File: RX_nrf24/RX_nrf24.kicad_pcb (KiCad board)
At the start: 2 copper layers, 58.5 x 26.2 mm, 44 parts, among them J1 USB_B_Micro, J2 Conn_01x03_Male, J3 Conn_Coaxial, J4 Conn_01x10_Male, J5 Conn_01x04_Female, J6 Conn_01x06_Male, J7 Conn_01x10_Male, J8 Conn_01x10_Male, SW1 SW_Push, U1 USBLC6-2SC6, U2 MCP1700-3302E_SOT23, U3 STM32F103C8Tx, U5 nRF24L01P, Y1 Crystal_GND24, Y2 Crystal_GND24

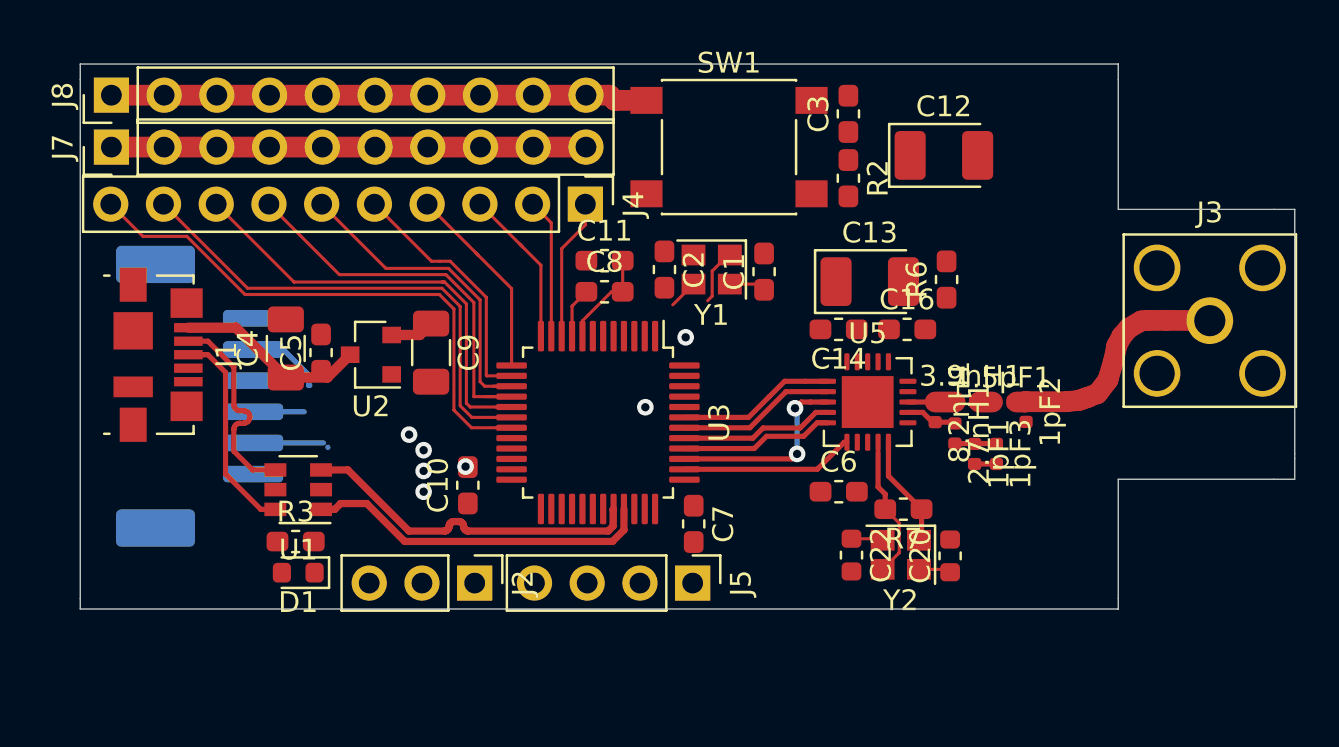
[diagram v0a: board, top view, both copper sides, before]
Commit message: update pcb
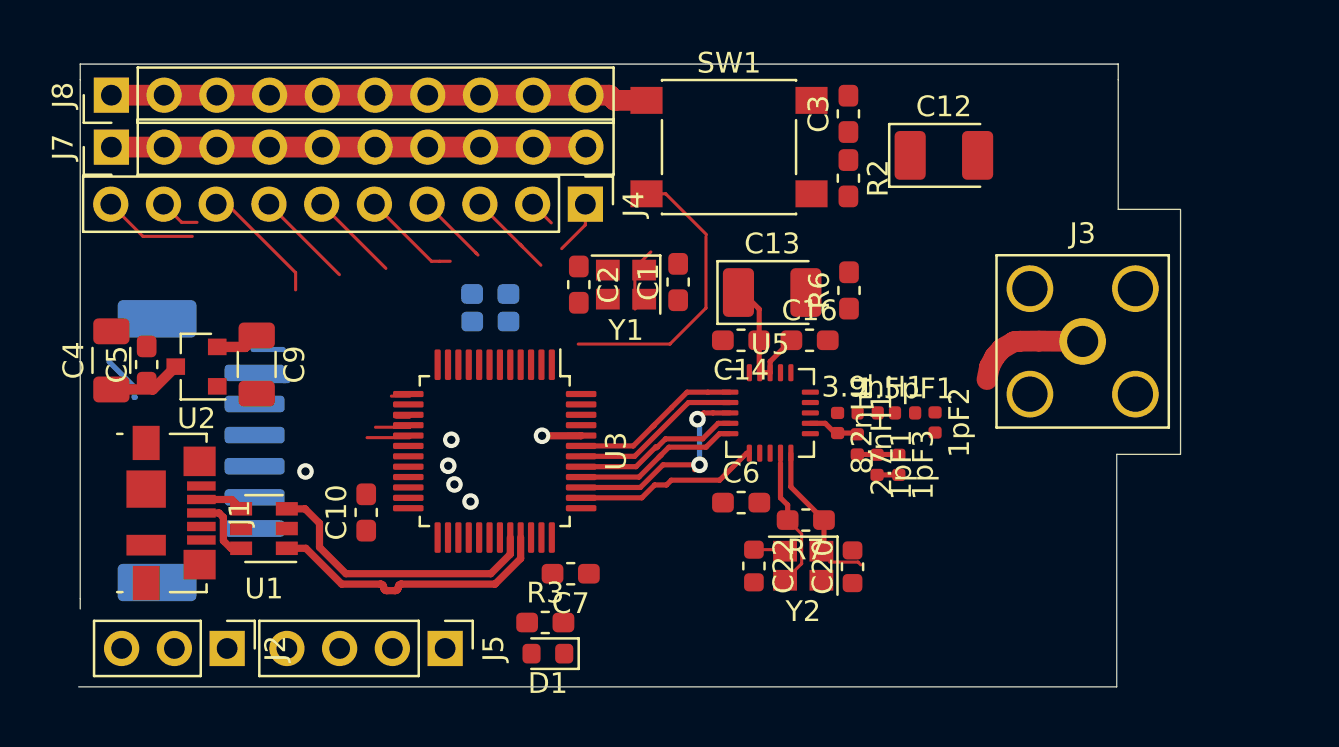
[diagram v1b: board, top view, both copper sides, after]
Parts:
- C11, C8: moved to B.Cu
- moved D1 12.6 mm to (172.5, 114.9)
- moved R3 12.6 mm to (172.4, 113.4)
- moved J2 12.3 mm to (157.1, 114.7)
- moved J5 12.3 mm to (167.6, 114.7)
- moved C4 8.42 mm to (151.5, 100.8)
- moved U2 8.42 mm to (155.6, 101.1)
- moved C5 8.42 mm to (153.2, 101.0)
- moved C9 8.42 mm to (158.5, 101.0)
- moved J1 7.65 mm to (154.4, 108.1)
- moved C7 6.39 mm to (173.6, 111.0), turned to 180 degrees
- moved C11 6.23 mm to (169.8, 98.9)
- moved J3 6.21 mm to (198.3, 99.9)
- moved C8 5.51 mm to (169.8, 97.6)
- moved U3 5.16 mm to (170.0, 105.1)
- moved C10 5.07 mm to (163.8, 108.1)
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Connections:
- U1 pad 2: Net-(U1-Pad2) -> GND
- U1 pad 5: Net-(U1-Pad5) -> +5V
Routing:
- net P10: track 27.4 -> 4.57 mm
- net P9: track 24.6 -> 1.98 mm
- net NRST: track 0.00 -> 14.0 mm
- net P8: track 21.9 -> 8.93 mm
- net P7: track 19.5 -> 7.19 mm
- net P6: track 16.0 -> 5.77 mm
- net D+: track 10.9 -> 3.28 mm
- net D-: track 10.1 -> 2.56 mm
- net P5: track 12.2 -> 4.79 mm
- net RF_out: track 12.0 -> 5.68 mm
- net +5V: track 9.24 -> 3.56 mm
- net P2: track 6.73 -> 1.27 mm
- net P4: track 9.60 -> 4.35 mm
- net +3V3: track 27.4 -> 31.9 mm
- net P1: track 7.49 -> 3.27 mm
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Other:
- board size 58.5 x 26.2 mm -> 53.1 x 30 mm
